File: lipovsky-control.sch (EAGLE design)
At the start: 46 parts, among them J1 JUMPER-PAD, P1 M04-929P, P2 M04-929P, P3 M04-929P, P4 M04-929P, U1 ATTINYX4A8MU, U2 MIC2288YD5, U3 MIC2288YD5, U4 LTV-816S

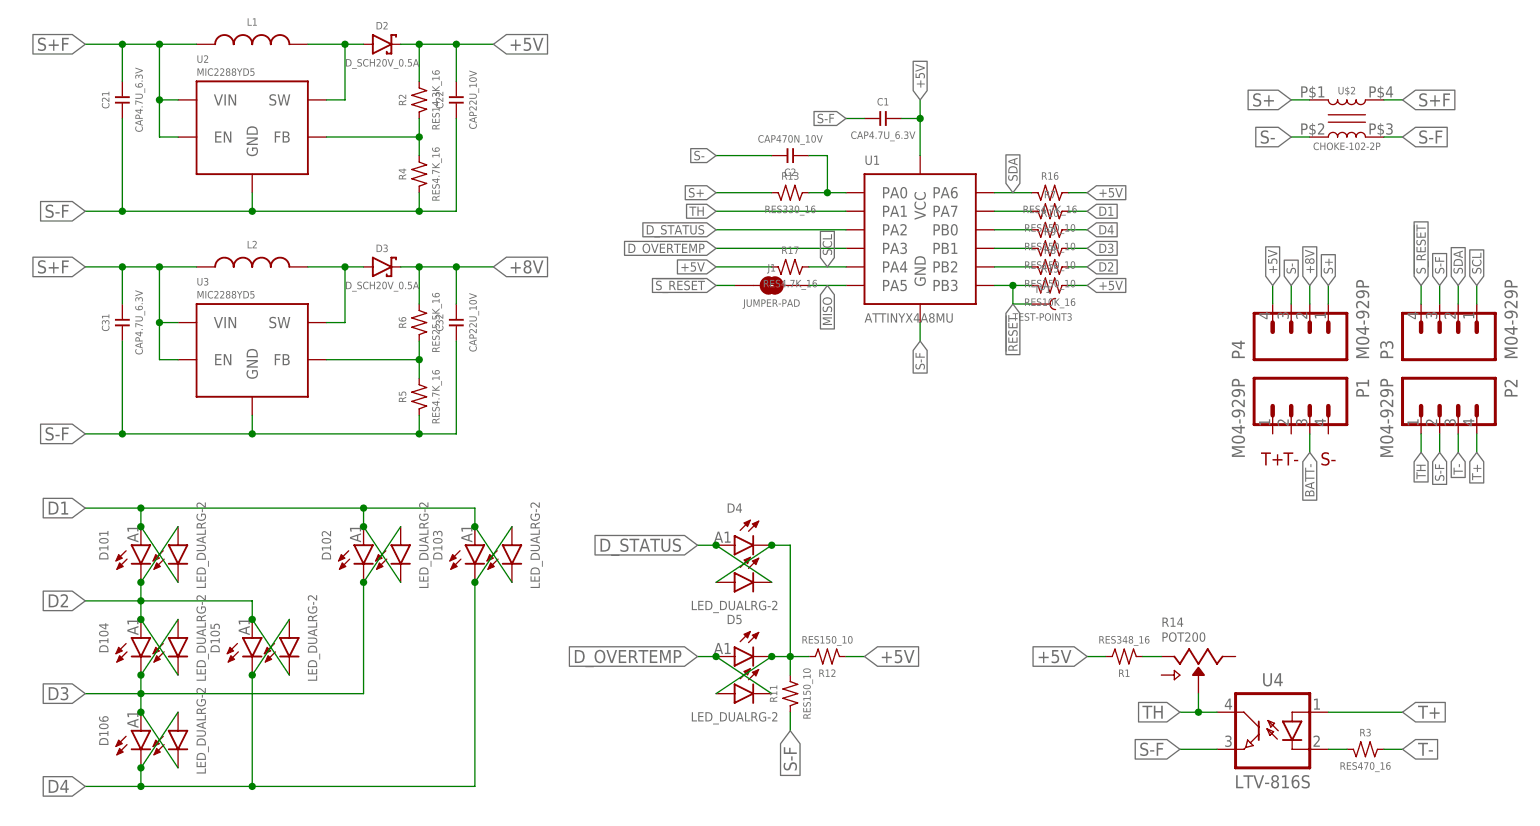
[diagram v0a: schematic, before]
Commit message: routing
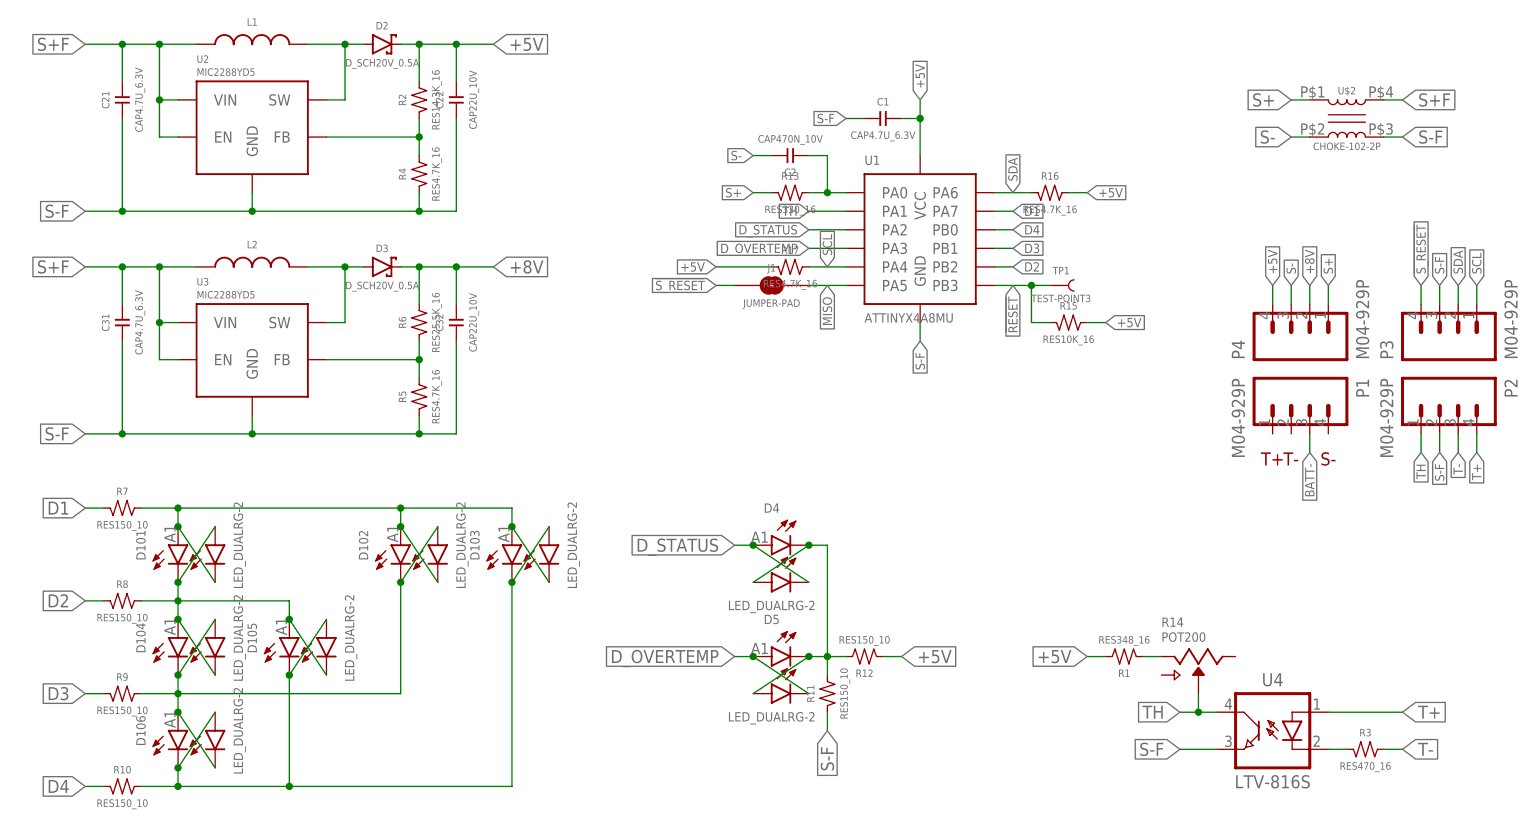
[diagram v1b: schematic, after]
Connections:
- removed net N$3: R10.1, U1.PB0
- removed net N$5: R8.1, U1.PB2
- removed net N$6: R7.1, U1.PA7
- removed net N$7: R9.1, U1.PB1
- new net D1L: D101.A1, D101.C2, D102.A1, D102.C2, D103.A1, D103.C2, R7.2
- new net D2L: D101.A2, D101.C1, D104.A1, D104.C2, D105.A1, D105.C2, R8.2
- new net D3L: D102.A2, D102.C1, D104.A2, D104.C1, D106.A1, D106.C2, R9.2
- new net D4L: D103.A2, D103.C1, D105.A2, D105.C1, D106.A2, D106.C1, R10.2
- net D1: now also R7.1, U1.PA7; no longer D101.A1, D101.C2, D102.A1, D102.C2, D103.A1, D103.C2, R7.2
- net D2: now also R8.1, U1.PB2; no longer D101.A2, D101.C1, D104.A1, D104.C2, D105.A1, D105.C2, R8.2
- net D3: now also R9.1, U1.PB1; no longer D102.A2, D102.C1, D104.A2, D104.C1, D106.A1, D106.C2, R9.2
- net D4: now also R10.1, U1.PB0; no longer D103.A2, D103.C1, D105.A2, D105.C1, D106.A2, D106.C1, R10.2
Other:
- moved on the sheet: D101, D102, D103, D104, D105, D106, D4, D5, R10, R11, R12, R15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
